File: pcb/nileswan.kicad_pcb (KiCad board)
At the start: 4 copper layers, 61.2 x 36.6 mm, 54 parts, among them J1 Micro_SD_Card_Det_Hirose_DM3AT, J2 Conn_01x06, U1 ICE40HX1K-VQ100, U2 W25Q16JVZPIQ, U3 AP2127N-1.2, U4 IS66WVE4M16EBLL-70BLI, Y1 AMPMAFB-25.0000T

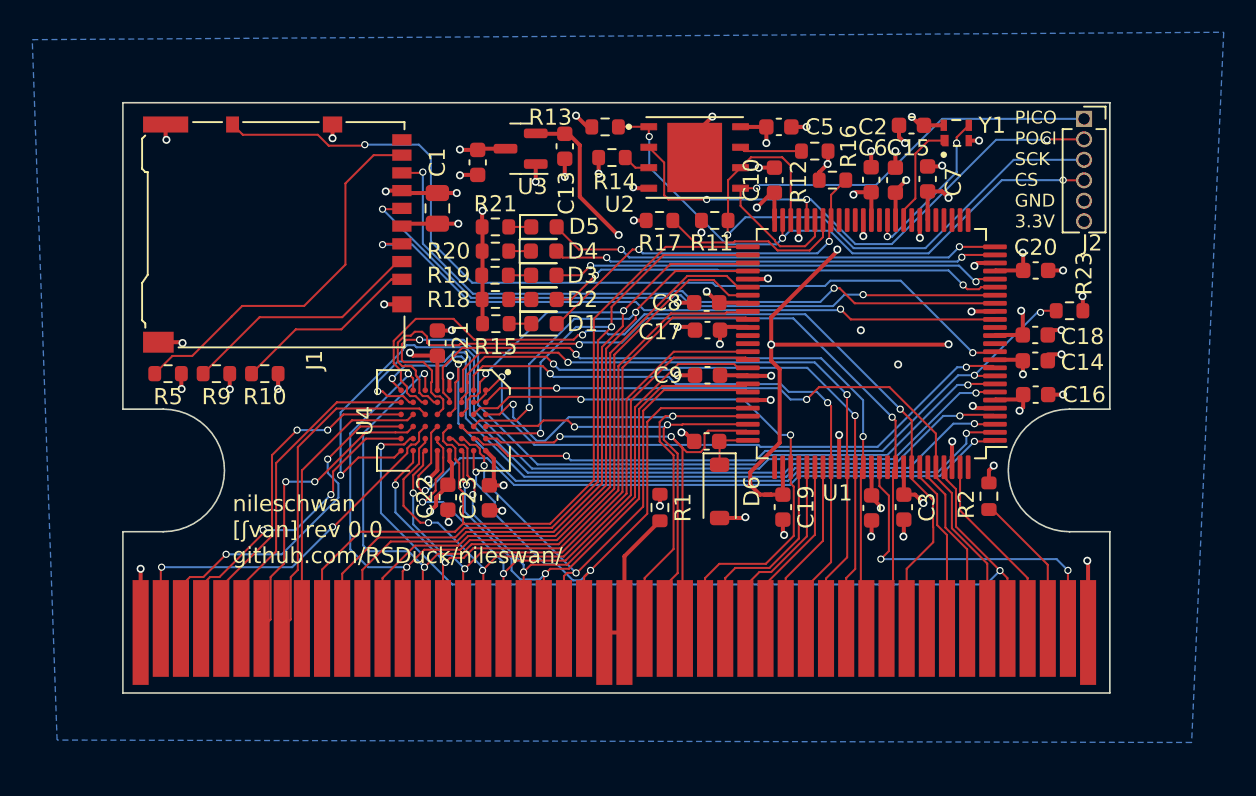
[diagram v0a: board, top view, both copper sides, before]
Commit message: second pcb iteration
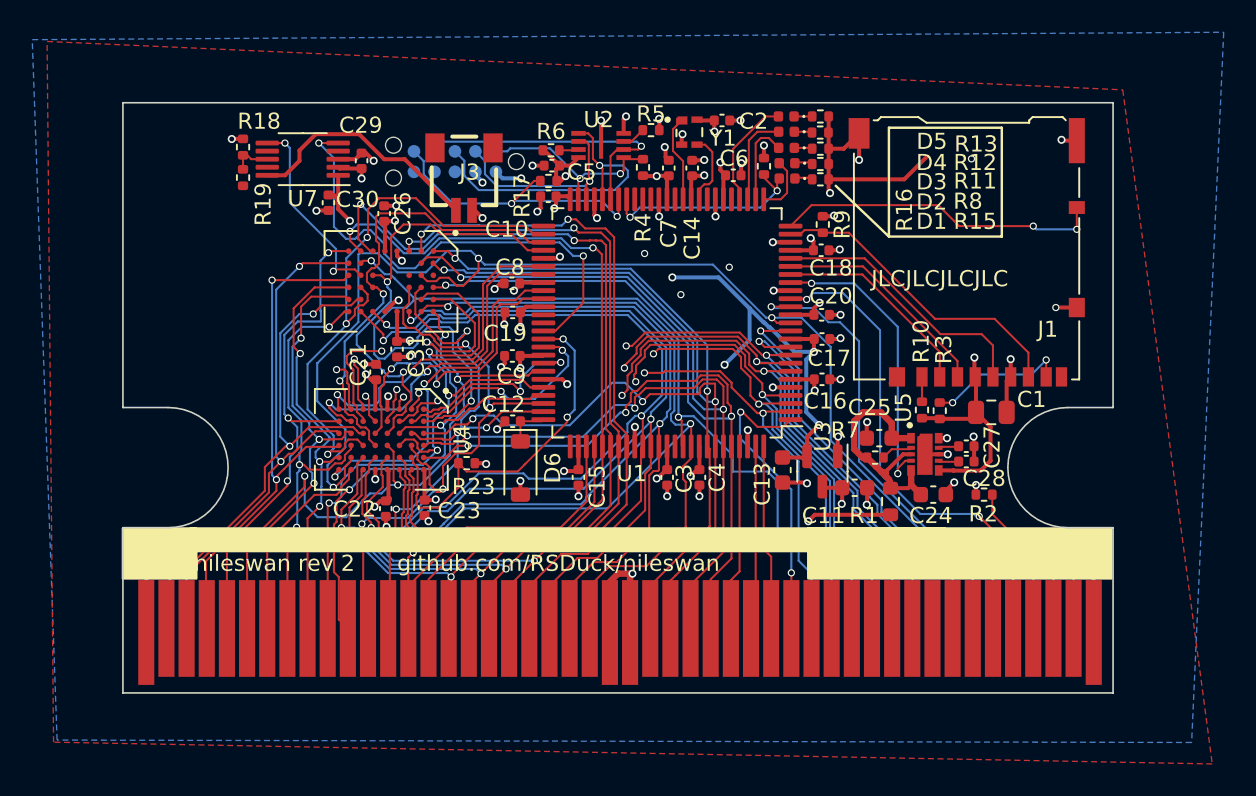
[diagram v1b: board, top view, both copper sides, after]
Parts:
- removed J2: Conn_01x06, Connector_PinSocket_1.27mm:PinSocket_1x06_P1.27mm_Vertical
- removed R14: 10k, Resistor_SMD:R_0603_1608Metric
- removed R20, R21: 2.2k, Resistor_SMD:R_0603_1608Metric
- added C24: 1 μF, Capacitor_SMD:C_0603_1608Metric, F.Cu at (163.1, 106.2)
- added C25: 1 μF, Capacitor_SMD:C_0603_1608Metric, F.Cu at (159.7, 102.7)
- added C26: 100 nF, Capacitor_SMD:C_0402_1005Metric, F.Cu at (129.0, 88.8)
- added C27: 470 pF, Capacitor_SMD:C_0402_1005Metric, F.Cu at (165.1, 103.2)
- added C28: 4.7 nF, Capacitor_SMD:C_0402_1005Metric, F.Cu at (165.1, 104.2)
- added C29: 100 nF, Capacitor_SMD:C_0402_1005Metric, F.Cu at (127.6, 85.5)
- added C30: 100 nF, Capacitor_SMD:C_0402_1005Metric, F.Cu at (125.5, 88.1)
- added C31: 100 nF, Capacitor_SMD:C_0402_1005Metric, F.Cu at (129.8, 97.2)
- added J3: SM02B-SRSS-TB_LF__SN_, snapeda:SM02B-SRSS-TB_LF__SN_, F.Cu at (133.9, 86.6)
- added J4: Conn_02x05_Counter_Clockwise, Connector:Tag-Connect_TC2050-IDC-NL_2x05_P1.27mm_Vertical, B.Cu at (133.4, 85.5)
- added R3: 47k, Resistor_SMD:R_0402_1005Metric, F.Cu at (163.4, 101.0)
- added R4: 10k, Resistor_SMD:R_0402_1005Metric, F.Cu at (145.1, 85.9)
- added R6: 10k, Resistor_SMD:R_0402_1005Metric, F.Cu at (139.3, 84.8)
- added R7: 10k, Resistor_SMD:R_0402_1005Metric, F.Cu at (159.4, 103.9)
- added R8: 2.2k, Resistor_SMD:R_0402_1005Metric, F.Cu at (156.1, 85.7)
- added U5: AP22966DC8-7, snapeda:IC_AP22966DC8-7, F.Cu at (162.5, 103.7)
- added U6: IS62WV5128EBLL-45BLI, nileswan:BGA-36_6x8_6.0x8.0mm, F.Cu at (129.4, 93.0)
- added U7: TPS3613, Package_SO:VSSOP-10_3x3mm_P0.5mm, F.Cu at (124.0, 85.4)
- C10, C12, C14, C15, C16, C17, C18, C19, C2, C20, C21, C22, C23, C3, C4, C5, C6, C7, C8, C9: footprint Capacitor_SMD:C_0603_1608Metric -> Capacitor_SMD:C_0402_1005Metric
- D1, D2, D3, D4, D5: footprint LED_SMD:LED_0603_1608Metric -> LED_SMD:LED_0402_1005Metric
- R10, R15, R16, R17, R2, R23, R9: footprint Resistor_SMD:R_0603_1608Metric -> Resistor_SMD:R_0402_1005Metric
- R11, R12, R13: value 10k -> 2.2k; footprint Resistor_SMD:R_0603_1608Metric -> Resistor_SMD:R_0402_1005Metric
- R18: value 2.2k -> 118k; footprint Resistor_SMD:R_0603_1608Metric -> Resistor_SMD:R_0402_1005Metric
- R19: value 2.2k -> 75k; footprint Resistor_SMD:R_0603_1608Metric -> Resistor_SMD:R_0402_1005Metric
- R5: value 47k -> 10k; footprint Resistor_SMD:R_0603_1608Metric -> Resistor_SMD:R_0402_1005Metric
- U2: value W25Q16JVZPIQ -> W25Q16JVUXIQ; footprint snapeda:SON127P500X600X80-9N -> snapeda:SON50P300X200X60-9N
- moved J1 42.8 mm to (165.1, 91.2), turned to 180 degrees
- moved R10 40.8 mm to (162.3, 101.0), turned to 90 degrees
- moved R9 38.7 mm to (156.2, 89.5), turned to -90 degrees
- moved R23 38.6 mm to (134.1, 104.2)
- moved C1 36.6 mm to (166.7, 101.1), turned to 0 degrees
- moved R5 33.5 mm to (145.6, 83.6)
- moved C11 30.9 mm to (158.2, 105.8), turned to 0 degrees
- moved U3 27.4 mm to (156.2, 104.8), turned to -90 degrees
- moved C15 26.9 mm to (141.1, 105.1), turned to -90 degrees
- moved C14 24.4 mm to (148.1, 86.0), turned to 90 degrees
- moved C13 24.2 mm to (153.7, 104.7)
- moved R15 22.0 mm to (156.1, 86.7)
- moved C19 20.7 mm to (137.0, 94.9), turned to 180 degrees
- moved R18 18.3 mm to (120.2, 84.7), turned to -90 degrees
- moved D1 17.6 mm to (154.0, 86.6), turned to 180 degrees
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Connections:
- net Net-(U1C-CRESET_B) renamed /fpga/CRESET_B
- net Net-(U3-VO) renamed 1.2V
- C1 pad 1: 3.3V -> 3.3V_TF
- J1 pad 10: /fpga/SD_DETECT -> /fpga/TF_DETECT
- J1 pad 2: Net-(J1-DAT3/CD) -> /fpga/TF_SEL
- J1 pad 3: /fpga/SD_CMD -> /fpga/TF_PICO
- J1 pad 4: 3.3V -> 3.3V_TF
- J1 pad 5: /fpga/SD_CLK -> /fpga/TF_CLK
- J1 pad 7: /fpga/SD_DAT0 -> /fpga/TF_POCI
- R1 pad 1: 3.3V -> Net-(U5-VBIAS)
- R10 pad 1: 3.3V -> 3.3V_TF
- R11 pad 1: 3.3V -> GND
- R11 pad 2: Net-(J2-Pin_3) -> Net-(D3-K)
- R12 pad 1: 3.3V -> GND
- R12 pad 2: Net-(U2-IO3) -> Net-(D4-K)
- R13 pad 1: 3.3V -> GND
- R13 pad 2: Net-(J2-Pin_4) -> Net-(D5-K)
- R15 pad 1: Net-(D1-K) -> GND
- R15 pad 2: GND -> Net-(D1-K)
- R18 pad 1: GND -> 3.3V
- R18 pad 2: Net-(D2-K) -> Net-(U7-SENSE)
- R19 pad 1: GND -> Net-(U7-SENSE)
- R19 pad 2: Net-(D3-K) -> GND
- R5 pad 2: Net-(J1-DAT1) -> Net-(U2-/WP)
- R9 pad 1: 3.3V -> 3.3V_TF
- R9 pad 2: Net-(J1-DAT3/CD) -> /fpga/TF_POCI
- U1 pad 1: /fpga/A_HIGH0 -> /fpga/A16
- U1 pad 10: /fpga/ENABLE_OUT_PSRAM -> /fpga/MBC
- U1 pad 100: unconnected-(U1A-IOT_95-Pad100) -> /fpga/A17
- U1 pad 12: /fpga/SD_DETECT -> /fpga//IO
- U1 pad 13: unconnected-(U1D-IOL_6B_GBIN7-Pad13) -> /fpga//WE
- U1 pad 15: unconnected-(U1D-IOL_7A_GBIN6-Pad15) -> /fpga/SCLK
- U1 pad 16: /fpga/SD_CMD -> /fpga//SEL
- U1 pad 18: /fpga/SD_DAT0 -> /fpga/TF_POW
- U1 pad 19: /fpga/SD_CLK -> /fpga/TF_SEL
- U1 pad 2: /fpga/A_HIGH1 -> /fpga/D8
- U1 pad 20: Net-(D2-A) -> /fpga/TF_PICO
- U1 pad 21: Net-(D3-A) -> /fpga/TF_CLK
- U1 pad 24: Net-(D4-A) -> /fpga/TF_POCI
- U1 pad 25: Net-(D5-A) -> /fpga/TF_DETECT
- U1 pad 26: unconnected-(U1C-IOB_26-Pad26) -> Net-(D2-A)
- U1 pad 27: unconnected-(U1C-IOB_27-Pad27) -> Net-(D3-A)
- U1 pad 28: unconnected-(U1C-IOB_28-Pad28) -> Net-(D4-A)
- U1 pad 29: unconnected-(U1C-IOB_29-Pad29) -> Net-(D5-A)
- U1 pad 3: /fpga/A_HIGH2 -> /fpga/D9
- U1 pad 4: /fpga/A_HIGH3 -> /fpga/D10
- U1 pad 45: Net-(J2-Pin_1) -> /fpga/FLASH_PICO
- U1 pad 46: Net-(J2-Pin_2) -> /fpga/FLASH_POCI
- U1 pad 48: Net-(J2-Pin_3) -> /fpga/FLASH_CLK
- U1 pad 49: Net-(J2-Pin_4) -> /fpga/FLASH_CS
- U1 pad 51: /fpga/A7 -> unconnected-(U1B-IOR_52-Pad51)
- U1 pad 52: /fpga/A6 -> /fpga/A_HIGH0
- U1 pad 53: /fpga/A5 -> /fpga/A_HIGH1
- U1 pad 54: /fpga/A4 -> /fpga/A_HIGH2
- U1 pad 56: /fpga/D15 -> /fpga/A_HIGH3
- U1 pad 57: /fpga/D14 -> /fpga/A_HIGH4
- U1 pad 59: /fpga/D7 -> /fpga/A_HIGH5
- U1 pad 60: /fpga/D6 -> /fpga/A_HIGH6
- U1 pad 64: /fpga/D5 -> /fpga//SEL_SRAM
- U1 pad 65: /fpga/D4 -> /fpga//SEL_PSRAM
- U1 pad 66: /fpga/D3 -> /fpga//PSRAM_UB
- U1 pad 68: /fpga/D2 -> /fpga//PSRAM_LB
- U1 pad 69: /fpga/D1 -> /fpga/A8
- U1 pad 7: /fpga/A_HIGH4 -> /fpga/D11
- U1 pad 71: /fpga/D0 -> /fpga/A7
- U1 pad 72: /fpga/A0 -> /fpga/A6
- U1 pad 73: /fpga/A1 -> /fpga/A5
- U1 pad 74: /fpga/A2 -> /fpga/A4
- U1 pad 78: /fpga/A3 -> /fpga/D15
- U1 pad 79: /fpga/A19 -> /fpga/D14
- U1 pad 8: /fpga/A_HIGH5 -> /fpga/D12
- U1 pad 80: /fpga/A18 -> /fpga/D7
- U1 pad 81: /fpga/A17 -> /fpga/D6
- U1 pad 82: /fpga/A16 -> /fpga/D5
- U1 pad 83: /fpga/D8 -> /fpga/D4
- U1 pad 85: /fpga/D9 -> /fpga/D3
- U1 pad 86: /fpga/D10 -> /fpga/D2
- U1 pad 87: /fpga/D11 -> /fpga/D1
- U1 pad 89: /fpga/SCLK -> unconnected-(U1A-IOT_84_GBIN1-Pad89)
- U1 pad 9: /fpga//SEL_PSRAM -> /fpga/D13
- U1 pad 90: unconnected-(U1A-IOT_85_GBIN0-Pad90) -> /fpga//OE
- U1 pad 91: /fpga/D12 -> /fpga/D0
- U1 pad 93: /fpga/D13 -> /fpga/A0
- U1 pad 94: /fpga/MBC -> /fpga/A1
- U1 pad 95: /fpga//IO -> /fpga/A2
- U1 pad 96: /fpga//OE -> /fpga/A3
- U1 pad 97: /fpga//WE -> /fpga/A19
- U1 pad 99: /fpga//SEL -> /fpga/A18
- U2 pad 1: Net-(J2-Pin_4) -> /fpga/FLASH_CS
- U2 pad 2: Net-(J2-Pin_2) -> /fpga/FLASH_PICO
- U2 pad 5: Net-(J2-Pin_1) -> /fpga/FLASH_POCI
- U2 pad 6: Net-(J2-Pin_3) -> /fpga/FLASH_CLK
- U4 pad A1: /fpga/ENABLE_OUT_PSRAM -> /fpga//PSRAM_LB
- U4 pad A3: /fpga/A0 -> /fpga/A1
- U4 pad A4: /fpga/A1 -> /fpga/A2
- U4 pad A5: /fpga/A2 -> /fpga/A3
- U4 pad B2: /fpga/ENABLE_OUT_PSRAM -> /fpga//PSRAM_UB
- U4 pad B3: /fpga/A3 -> /fpga/A4
- U4 pad B4: /fpga/A4 -> /fpga/A5
- U4 pad C3: /fpga/A5 -> /fpga/A6
- U4 pad C4: /fpga/A6 -> /fpga/A7
- U4 pad D3: /fpga/A_HIGH1 -> /fpga/A_HIGH2
- U4 pad D4: /fpga/A7 -> /fpga/A8
- U4 pad E3: /fpga/A_HIGH5 -> /fpga/A_HIGH6
- U4 pad E4: /fpga/A_HIGH0 -> /fpga/A_HIGH1
- U4 pad F3: /fpga/A14 -> /fpga/A15
- U4 pad F4: /fpga/A15 -> /fpga/A_HIGH0
- U4 pad G2: /fpga/A_HIGH3 -> /fpga/A_HIGH4
- U4 pad G3: /fpga/A12 -> /fpga/A13
- U4 pad G4: /fpga/A13 -> /fpga/A14
- U4 pad H1: /fpga/A_HIGH2 -> /fpga/A_HIGH3
- U4 pad H2: /fpga/A8 -> /fpga/A9
- U4 pad H3: /fpga/A9 -> /fpga/A10
- U4 pad H4: /fpga/A10 -> /fpga/A11
- U4 pad H5: /fpga/A11 -> /fpga/A12
- U4 pad H6: /fpga/A_HIGH4 -> /fpga/A_HIGH5
- Y1 pad 1: Net-(U1C-IOB_36_GBIN4) -> Net-(U1C-IOB_34)
- Y1 pad 3: Net-(U1C-IOB_34) -> Net-(U1C-IOB_36_GBIN4)
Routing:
- net /fpga/SD_DETECT: track 56.6 -> 0.00 mm, vias 2 -> 0
- net /fpga/SD_DAT0: track 43.8 -> 0.00 mm, vias 2 -> 0
- net /fpga/SD_CLK: track 42.1 -> 0.00 mm, vias 2 -> 0
- net /fpga/SD_CMD: track 41.2 -> 0.00 mm, vias 2 -> 0
- net /fpga/ENABLE_OUT_PSRAM: track 38.4 -> 0.00 mm, vias 2 -> 0
- net Net-(J2-Pin_4): track 37.1 -> 0.00 mm, vias 3 -> 0
- net Net-(J2-Pin_3): track 37.1 -> 0.00 mm, vias 1 -> 0
- net /fpga/A_HIGH4: track 57.7 -> 21.9 mm
- net /fpga//OE: track 43.5 -> 78.2 mm, vias 2 -> 4
- net Net-(J2-Pin_2): track 34.6 -> 0.00 mm, vias 3 -> 0
- net /fpga/D0: track 35.0 -> 67.9 mm, vias 2 -> 3
- net /fpga/D3: track 36.7 -> 68.9 mm, vias 2 -> 3
- net /fpga/A2: track 30.3 -> 61.9 mm, vias 2 -> 4
- net /fpga//SEL_SRAM: track 0.00 -> 31.2 mm, vias 0 -> 2
- net Net-(J2-Pin_1): track 31.1 -> 0.00 mm, vias 1 -> 0
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- added copper zone on F.Cu, net GND
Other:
- board size 61.2 x 36.6 mm -> 61.4 x 36.6 mm
- board text added: "JLCJLCJLCJLC"
- board text added: "nileswan rev 2 github.com/RSDuck/nileswan"
- board text removed: "PICO POCI SCK CS GND 3.3V"
- board text removed: "nileschwan [ʃvan] rev 0.0 github.com/RSDuck/nileswan/"
